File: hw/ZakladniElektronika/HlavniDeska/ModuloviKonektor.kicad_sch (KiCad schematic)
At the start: 1 part, among them J4 Conn_01x07

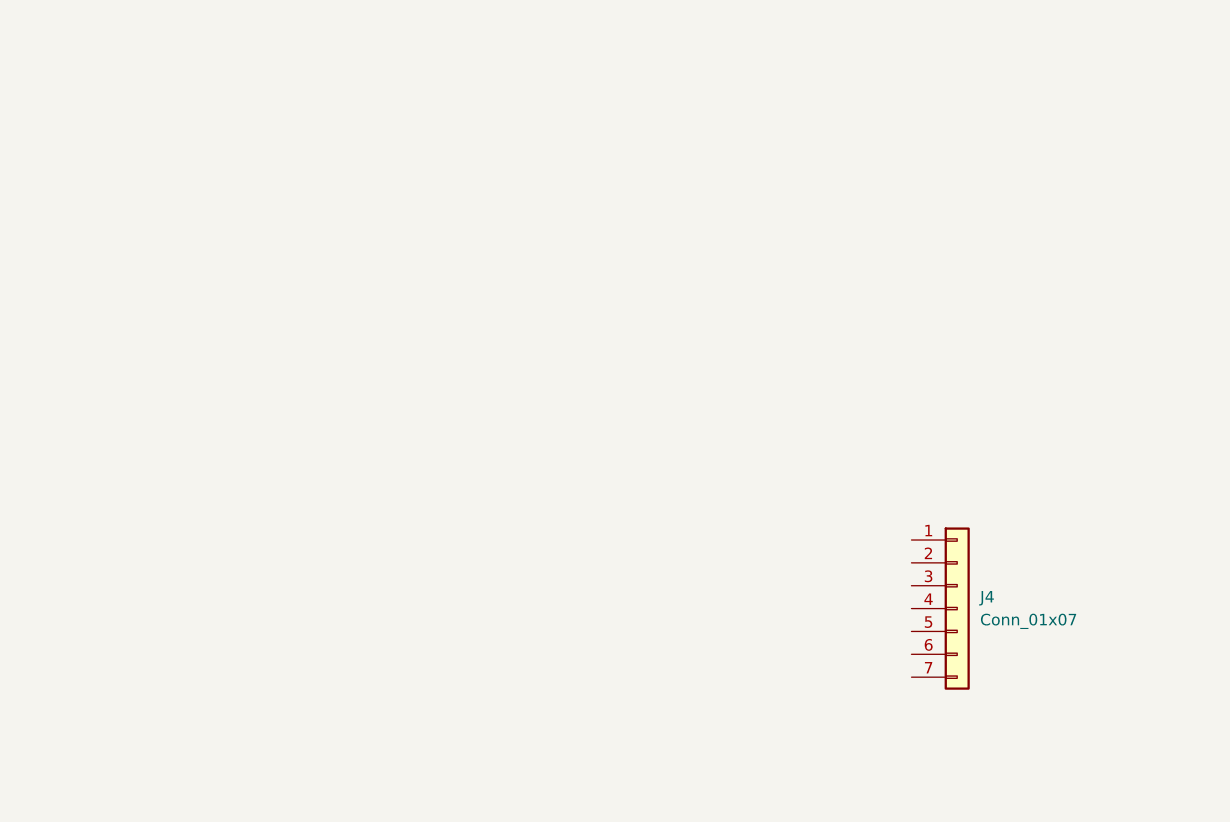
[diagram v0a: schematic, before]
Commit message: Nastin schematu
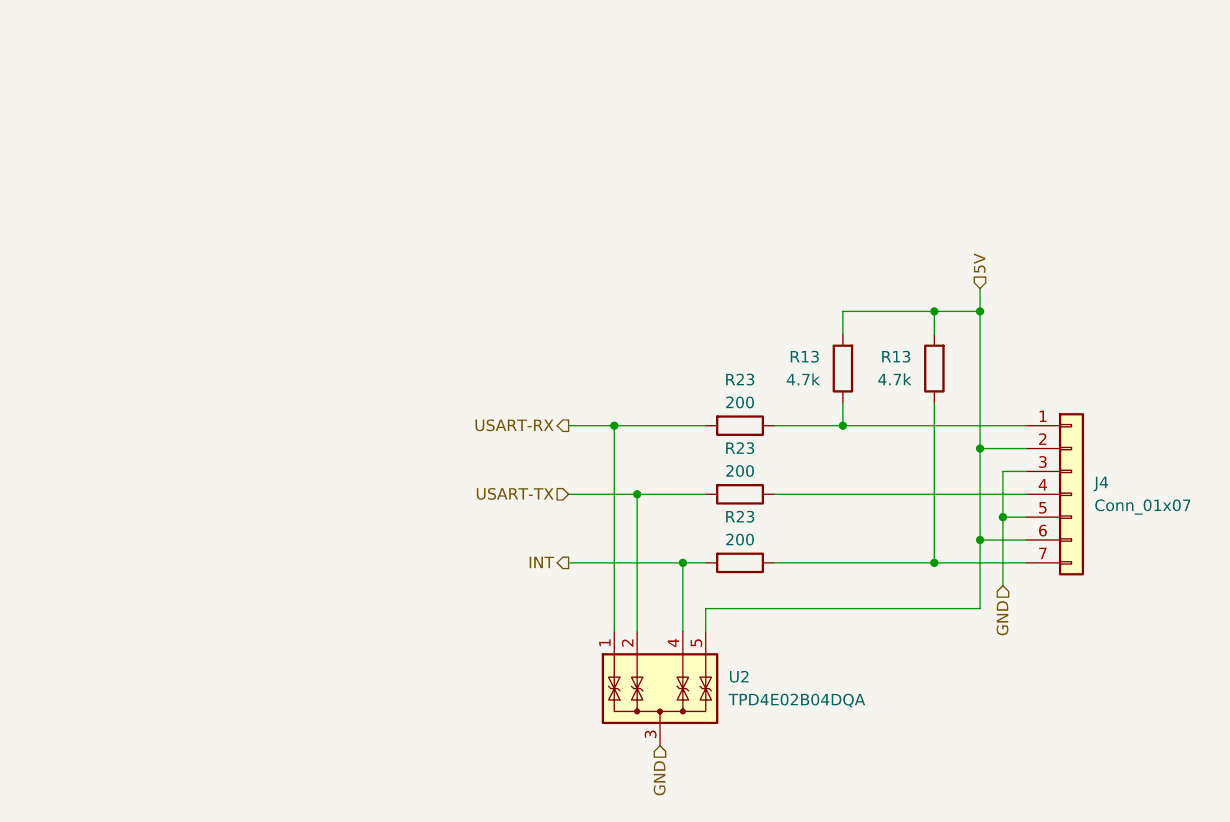
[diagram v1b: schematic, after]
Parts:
- added R13 (x2): 4.7k, Resistor_SMD:R_0201_0603Metric, symbol Device:R
- added R23 (x3): 200, Resistor_SMD:R_0402_1005Metric, symbol Device:R
- added U2: TPD4E02B04DQA, Package_SON:USON-10_2.5x1.0mm_P0.5mm, symbol Power_Protection:TPD4E02B04DQA
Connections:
- net at J4.1 (Pin_1): now also R13.1, R23.1
- net 5V: now reaches J4.2 (Pin_2)
- net 5V: now also J4.6 (Pin_6), R13.2, R13.2, U2.5 (IO4)
- net GND: now reaches J4.3 (Pin_3)
- net GND: now also J4.5 (Pin_5), U2.3 (G), U2.8 (G)
- net at J4.4 (Pin_4): now also R23.1
- net at J4.7 (Pin_7): now also R13.1, R23.1
- new net INT: R23.2, U2.4 (IO3)
- new net USART-RX: R23.2, U2.1 (IO1)
- new net USART-TX: R23.2, U2.2 (IO2)
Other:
- moved on the sheet: J4

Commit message: WIP
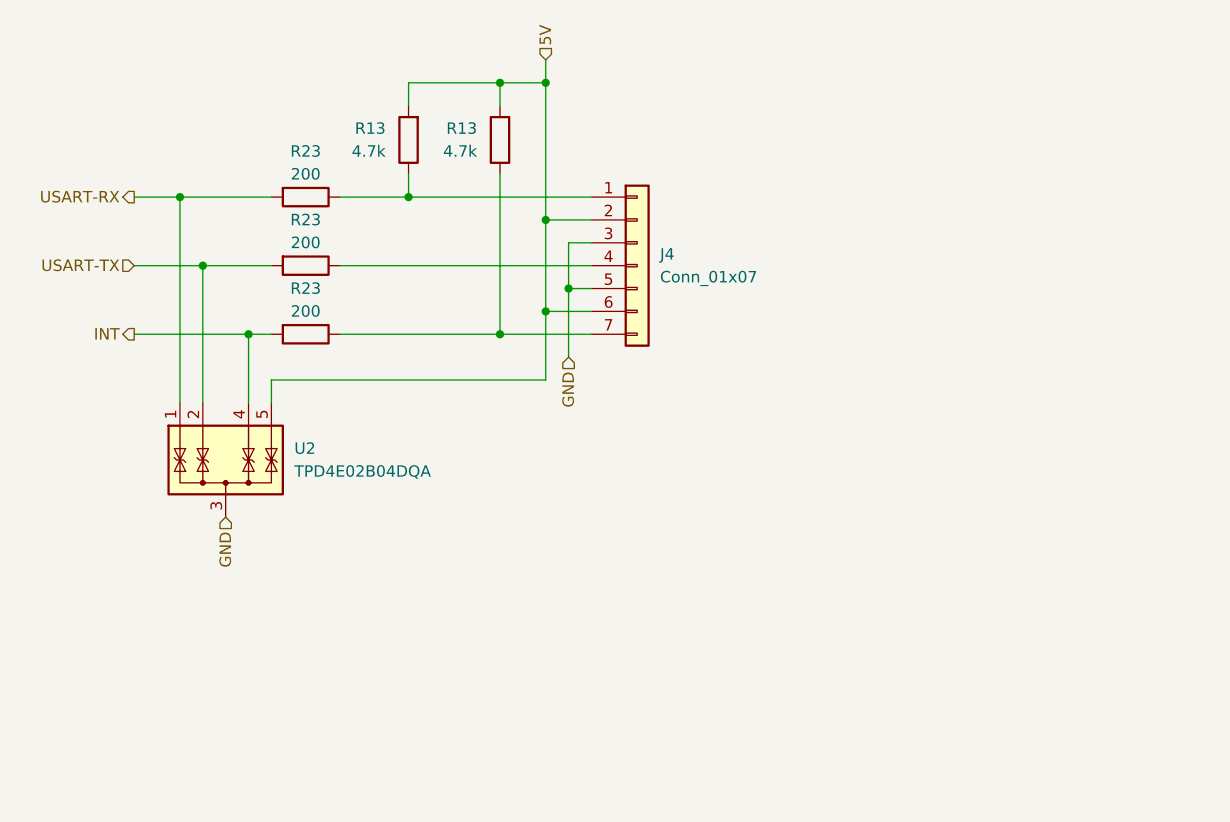
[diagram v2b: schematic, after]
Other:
- moved on the sheet: J4, R13, R23, U2
